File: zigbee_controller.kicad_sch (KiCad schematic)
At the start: 73 parts, among them J1 KF635, J10 TerminalBlock_KF301-5.0, J11 TerminalBlock_KF301-5.0, J12 TerminalBlock_KF301-5.0, J13 TerminalBlock_KF301-5.0, J3 Conn_01x06, J4 Conn_01x07, J5 Conn_01x05, P1 USB_C_Receptacle_GCT_USB4105, Q2 IRLB3813, Q3 IRLB3813, Q4 IRLB3813, Q5 IRLB3813, SW2 EN, SW4 Boot, U1 TPS54560, U2 ESP32-C6-MINI-1, U4 TC4427, U5 TC4427, U6 RT9080, U9 CH224K

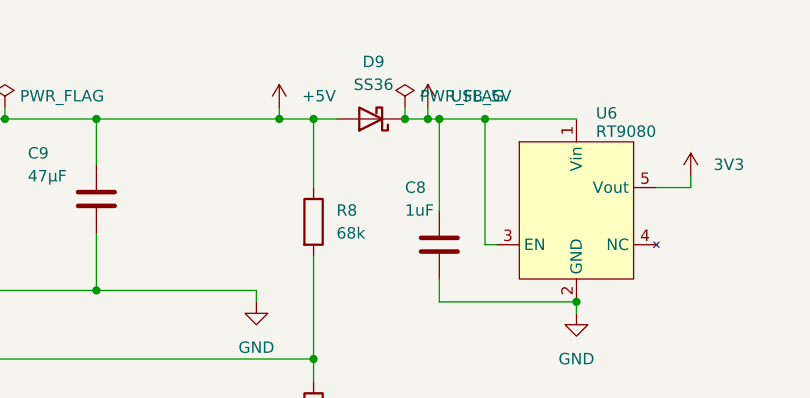
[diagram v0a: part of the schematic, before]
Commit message: Final rev2
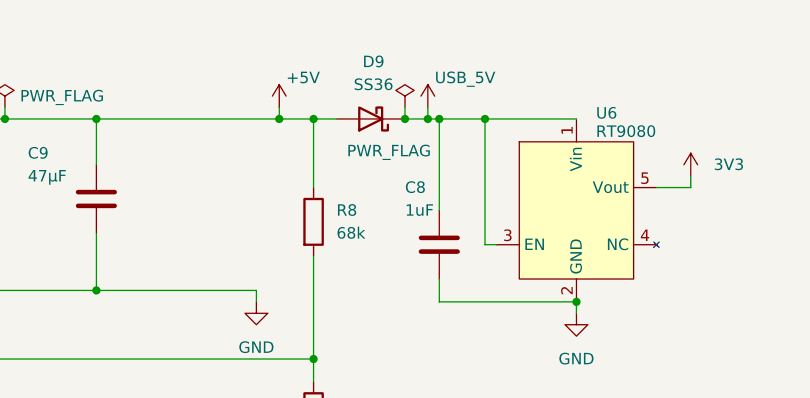
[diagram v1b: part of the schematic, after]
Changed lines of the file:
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@@
 		(in_pos_files yes)
 		(dnp no)
-		(fields_autoplaced yes)
 		(property "Reference" "#PWR045"
 			(at 248.92 26.67 0)
@@
 		)
 		(property "Value" "USB_5V"
-			(at 251.46 21.5899 0)
+			(at 249.682 19.558 0)
 			(show_name no)
 			(do_not_autoplace no)
@@
 		)
 		(property "Value" "PWR_FLAG"
-			(at 252.73 21.59 0)
+			(at 244.602 27.686 0)
 			(show_name no)
 			(do_not_autoplace no)
@@
 		(in_pos_files yes)
 		(dnp no)
-		(fields_autoplaced yes)
 		(property "Reference" "#PWR09"
 			(at 232.41 26.67 0)
@@
 		)
 		(property "Value" "+5V"
-			(at 234.95 21.5899 0)
+			(at 233.172 19.558 0)
 			(show_name no)
 			(do_not_autoplace no)
